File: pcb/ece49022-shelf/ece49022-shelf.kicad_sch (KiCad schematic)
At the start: 0 parts

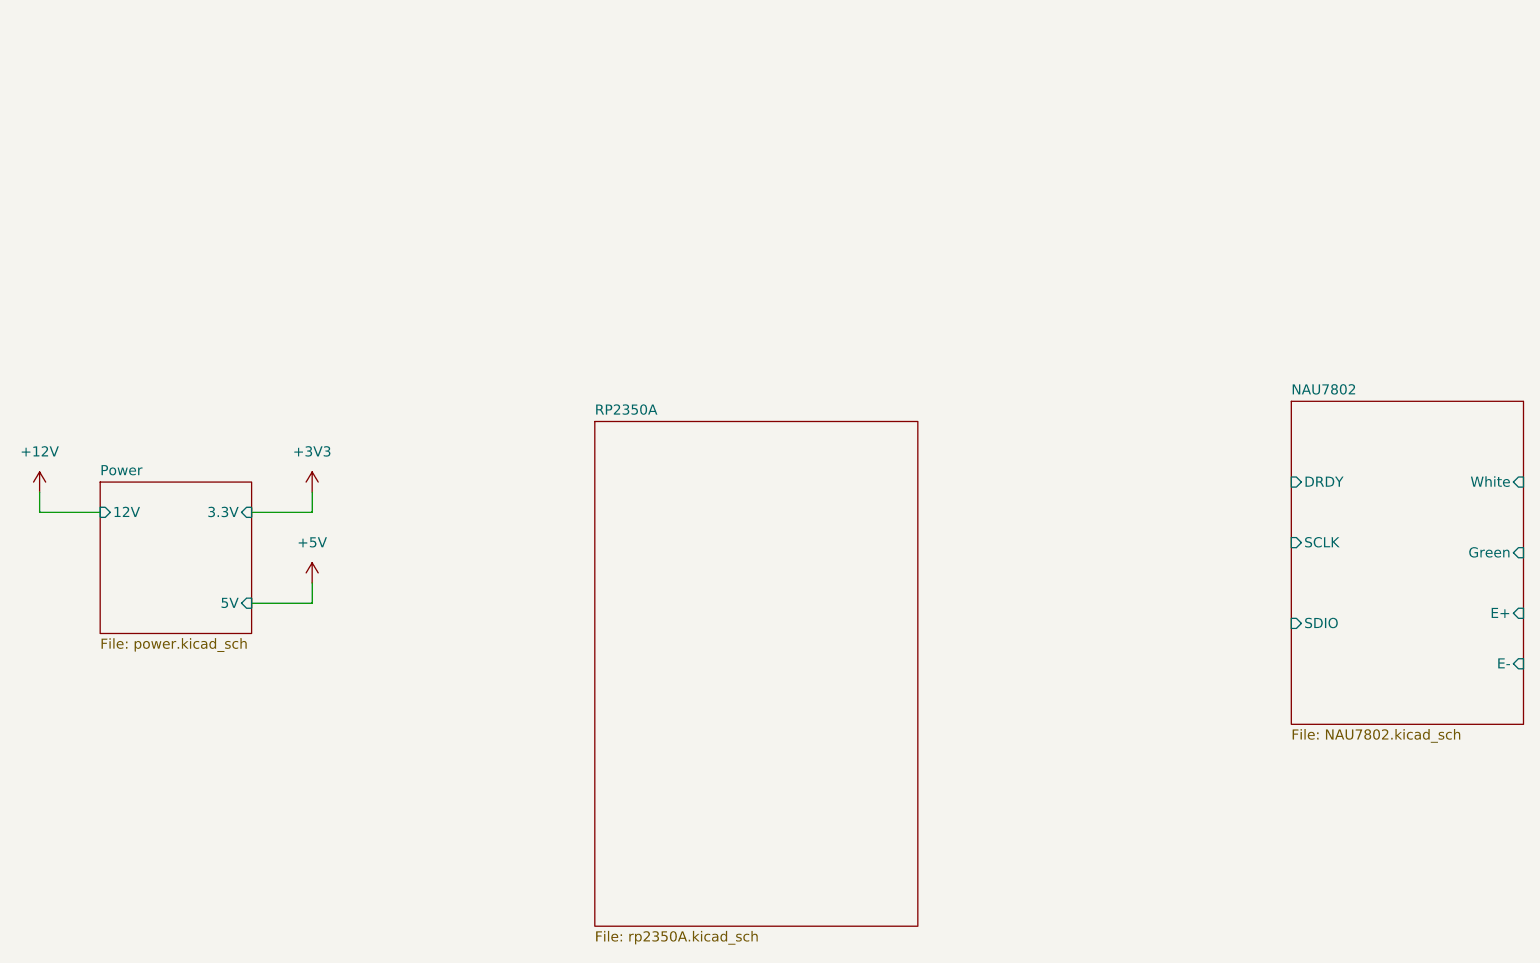
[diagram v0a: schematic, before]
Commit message: quicksave
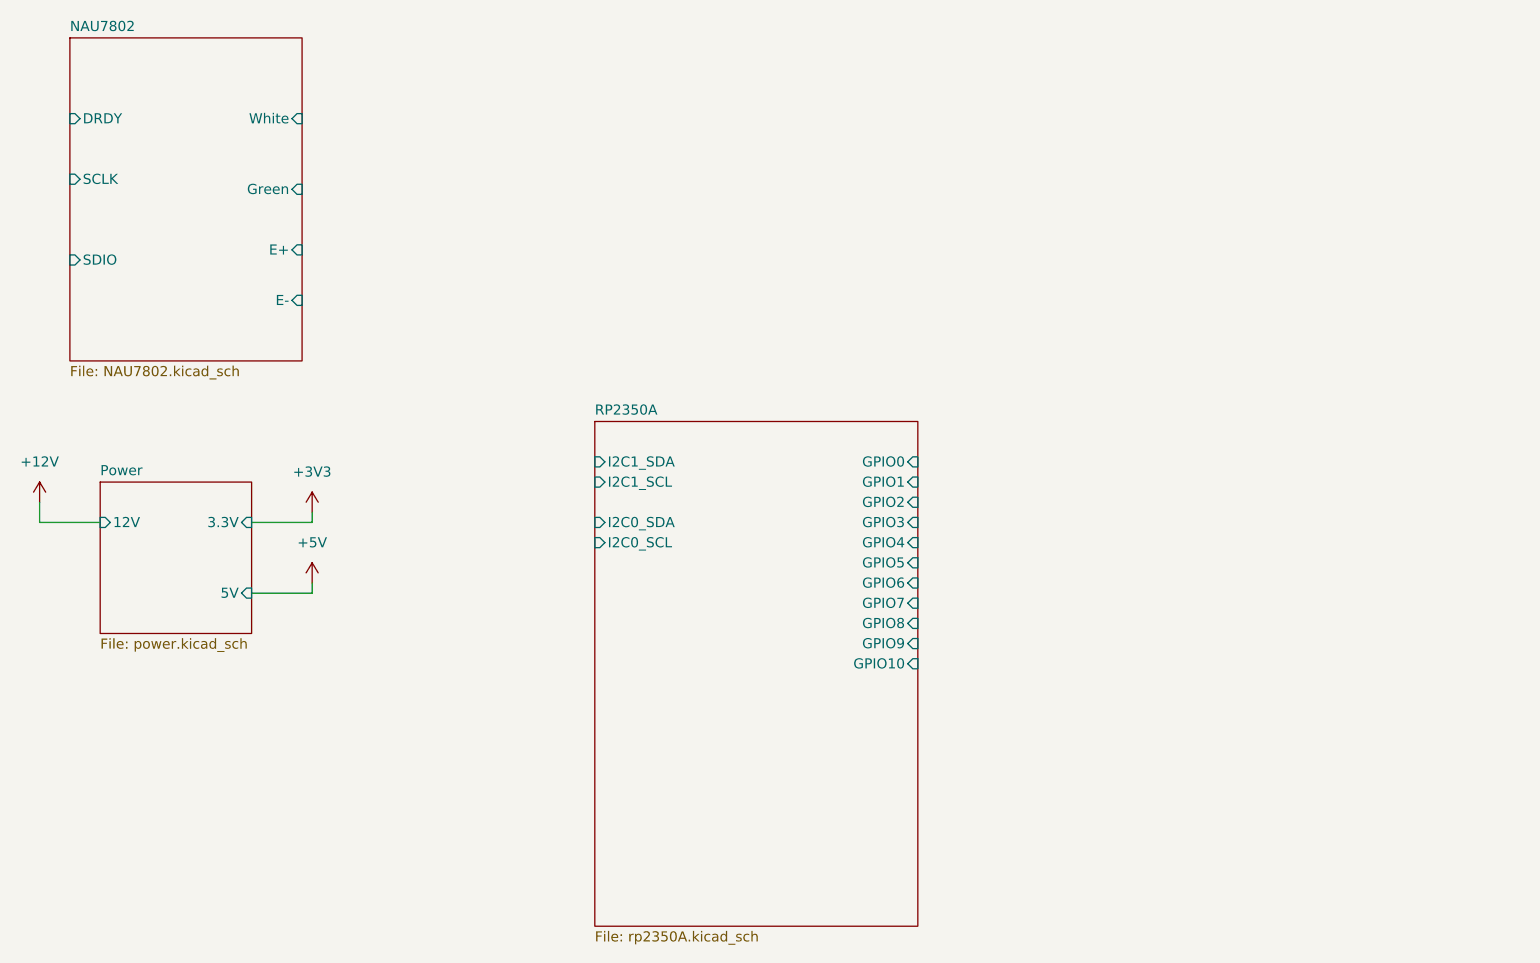
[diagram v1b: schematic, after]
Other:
- sheet RP2350A ports: added GPIO0, GPIO1, GPIO10, GPIO2, GPIO3, GPIO4, GPIO5, GPIO6, GPIO7, GPIO8, GPIO9, I2C0_SCL, I2C0_SDA, I2C1_SCL, I2C1_SDA; removed none
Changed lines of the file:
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@@
 	(wire
 		(pts
-			(xy 52.07 97.79) (xy 59.69 97.79)
+			(xy 52.07 96.52) (xy 59.69 96.52)
 		)
 		(stroke
@@
 	(wire
 		(pts
-			(xy 59.69 95.25) (xy 59.69 97.79)
+			(xy 59.69 96.52) (xy 59.69 95.25)
 		)
 		(stroke
@@
 	(wire
 		(pts
-			(xy 59.69 83.82) (xy 59.69 86.36)
+			(xy 59.69 86.36) (xy 59.69 87.63)
 		)
 		(stroke
@@
 	(wire
 		(pts
-			(xy 52.07 86.36) (xy 59.69 86.36)
+			(xy 52.07 87.63) (xy 59.69 87.63)
 		)
 		(stroke
@@
 	(wire
 		(pts
-			(xy 25.4 83.82) (xy 25.4 86.36)
+			(xy 25.4 85.09) (xy 25.4 87.63)
 		)
 		(stroke
@@
 	(wire
 		(pts
-			(xy 33.02 86.36) (xy 25.4 86.36)
+			(xy 33.02 87.63) (xy 25.4 87.63)
 		)
 		(stroke
@@
 	(symbol
 		(lib_id "power:+3V3")
-		(at 59.69 83.82 0)
+		(at 59.69 86.36 0)
 		(unit 1)
 		(exclude_from_sim no)
@@
 		(fields_autoplaced yes)
 		(property "Reference" "#PWR012"
-			(at 59.69 87.63 0)
+			(at 59.69 90.17 0)
 			(effects
 				(font
@@
 		)
 		(property "Value" "+3V3"
-			(at 59.69 78.74 0)
+			(at 59.69 81.28 0)
 			(effects
 				(font
@@
 		)
 		(property "Footprint" ""
-			(at 59.69 83.82 0)
+			(at 59.69 86.36 0)
 			(effects
 				(font
@@
 		)
 		(property "Datasheet" ""
-			(at 59.69 83.82 0)
+			(at 59.69 86.36 0)
 			(effects
 				(font
@@
 		)
 		(property "Description" "Power symbol creates a global label with name \"+3V3\""
-			(at 59.69 83.82 0)
+			(at 59.69 86.36 0)
 			(effects
 				(font
@@
 	(symbol
 		(lib_id "power:+12V")
-		(at 25.4 83.82 0)
+		(at 25.4 85.09 0)
 		(unit 1)
 		(exclude_from_sim no)
@@
 		(fields_autoplaced yes)
 		(property "Reference" "#PWR011"
-			(at 25.4 87.63 0)
+			(at 25.4 88.9 0)
 			(effects
 				(font
@@
 		)
 		(property "Value" "+12V"
-			(at 25.4 78.74 0)
+			(at 25.4 80.01 0)
 			(effects
 				(font
@@
 		)
 		(property "Footprint" ""
-			(at 25.4 83.82 0)
+			(at 25.4 85.09 0)
 			(effects
 				(font
@@
 		)
 		(property "Datasheet" ""
-			(at 25.4 83.82 0)
+			(at 25.4 85.09 0)
 			(effects
 				(font
@@
 		)
 		(property "Description" "Power symbol creates a global label with name \"+12V\""
-			(at 25.4 83.82 0)
+			(at 25.4 85.09 0)
 			(effects
 				(font
@@
 		)
 		(pin "5V" input
-			(at 52.07 97.79 0)
+			(at 52.07 96.52 0)
 			(effects
 				(font
@@
 		)
 		(pin "3.3V" input
-			(at 52.07 86.36 0)
+			(at 52.07 87.63 0)
 			(effects
 				(font
@@
 		)
 		(pin "12V" input
-			(at 33.02 86.36 180)
+			(at 33.02 87.63 180)
 			(effects
 				(font
@@
 			)
 		)
+		(pin "GPIO7" input
+			(at 135.89 97.79 0)
+			(effects
+				(font
+					(size 1.27 1.27)
+				)
+				(justify right)
+			)
+		)
+		(pin "I2C1_SDA" input
+			(at 95.25 80.01 180)
+			(effects
+				(font
+					(size 1.27 1.27)
+				)
+				(justify left)
+			)
+		)
+		(pin "GPIO2" input
+			(at 135.89 85.09 0)
+			(effects
+				(font
+					(size 1.27 1.27)
+				)
+				(justify right)
+			)
+		)
+		(pin "GPIO8" input
+			(at 135.89 100.33 0)
+			(effects
+				(font
+					(size 1.27 1.27)
+				)
+				(justify right)
+			)
+		)
+		(pin "GPIO3" input
+			(at 135.89 87.63 0)
+			(effects
+				(font
+					(size 1.27 1.27)
+				)
+				(justify right)
+			)
+		)
+		(pin "GPIO0" input
+			(at 135.89 80.01 0)
+			(effects
+				(font
+					(size 1.27 1.27)
+				)
+				(justify right)
+			)
+		)
+		(pin "GPIO1" input
+			(at 135.89 82.55 0)
+			(effects
+				(font
+					(size 1.27 1.27)
+				)
+				(justify right)
+			)
+		)
+		(pin "GPIO5" input
+			(at 135.89 92.71 0)
+			(effects
+				(font
+					(size 1.27 1.27)
+				)
+				(justify right)
+			)
+		)
+		(pin "GPIO9" input
+			(at 135.89 102.87 0)
+			(effects
+				(font
+					(size 1.27 1.27)
+				)
+				(justify right)
+			)
+		)
+		(pin "I2C1_SCL" input
+			(at 95.25 82.55 180)
+			(effects
+				(font
+					(size 1.27 1.27)
+				)
+				(justify left)
+			)
+		)
+		(pin "GPIO4" input
+			(at 135.89 90.17 0)
+			(effects
+				(font
+					(size 1.27 1.27)
+				)
+				(justify right)
+			)
+		)
+		(pin "GPIO10" input
+			(at 135.89 105.41 0)
+			(effects
+				(font
+					(size 1.27 1.27)
+				)
+				(justify right)
+			)
+		)
+		(pin "GPIO6" input
+			(at 135.89 95.25 0)
+			(effects
+				(font
+					(size 1.27 1.27)
+				)
+				(justify right)
+			)
+		)
+		(pin "I2C0_SDA" input
+			(at 95.25 87.63 180)
+			(effects
+				(font
+					(size 1.27 1.27)
+				)
+				(justify left)
+			)
+		)
+		(pin "I2C0_SCL" input
+			(at 95.25 90.17 180)
+			(effects
+				(font
+					(size 1.27 1.27)
+				)
+				(justify left)
+			)
+		)
 		(instances
 			(project "ece49022-shelf"
@@
 	)
 	(sheet
-		(at 182.88 72.39)
+		(at 29.21 26.67)
 		(size 29.21 40.64)
 		(exclude_from_sim no)
@@
 		)
 		(property "Sheetname" "NAU7802"
-			(at 182.88 71.6784 0)
+			(at 29.21 25.9584 0)
 			(effects
 				(font
@@
 		)
 		(property "Sheetfile" "NAU7802.kicad_sch"
-			(at 182.88 113.6146 0)
+			(at 29.21 67.8946 0)
 			(effects
 				(font
@@
 		)
 		(pin "E-" input
-			(at 212.09 105.41 0)
+			(at 58.42 59.69 0)
 			(effects
 				(font
@@
 		)
 		(pin "E+" input
-			(at 212.09 99.06 0)
+			(at 58.42 53.34 0)
 			(effects
 				(font
@@
 		)
 		(pin "Green" input
-			(at 212.09 91.44 0)
+			(at 58.42 45.72 0)
 			(effects
 				(font
@@
 		)
 		(pin "White" input
-			(at 212.09 82.55 0)
+			(at 58.42 36.83 0)
 			(effects
 				(font
@@
 		)
 		(pin "DRDY" input
-			(at 182.88 82.55 180)
+			(at 29.21 36.83 180)
 			(effects
 				(font
@@
 		)
 		(pin "SCLK" input
-			(at 182.88 90.17 180)
+			(at 29.21 44.45 180)
 			(effects
 				(font
@@
 		)
 		(pin "SDIO" input
-			(at 182.88 100.33 180)
-			(effects
-				(font
+			(at 29.21 54.61 180)
+			(effects
+				(font
